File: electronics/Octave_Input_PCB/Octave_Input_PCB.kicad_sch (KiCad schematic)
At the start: 66 parts, among them J1 HRO_TYPE-C-31-M-12, SW1 SW_Hot_Swap_Socket, SW10 SW_Hot_Swap_Socket, SW11 SW_Hot_Swap_Socket, SW12 SW_Hot_Swap_Socket, SW13 SW_Hot_Swap_Socket, SW14 Alps_Alpine_RKJXV1224, SW15 Bourns_PEC12R-4xxxF-Sxxx, SW2 SW_Hot_Swap_Socket, SW21 Alps_Alpine_SKRP, SW22 Alps_Alpine_SKRP, SW3 SW_Hot_Swap_Socket, SW4 SW_Hot_Swap_Socket, SW5 SW_Hot_Swap_Socket, SW6 SW_Hot_Swap_Socket, SW7 SW_Hot_Swap_Socket, SW8 SW_Hot_Swap_Socket, SW9 SW_Hot_Swap_Socket, U1 AP2112K-3.3, U2 Raspberry_Pi_RP2040, U3 W25Q64JVSS, Y1 12MHz

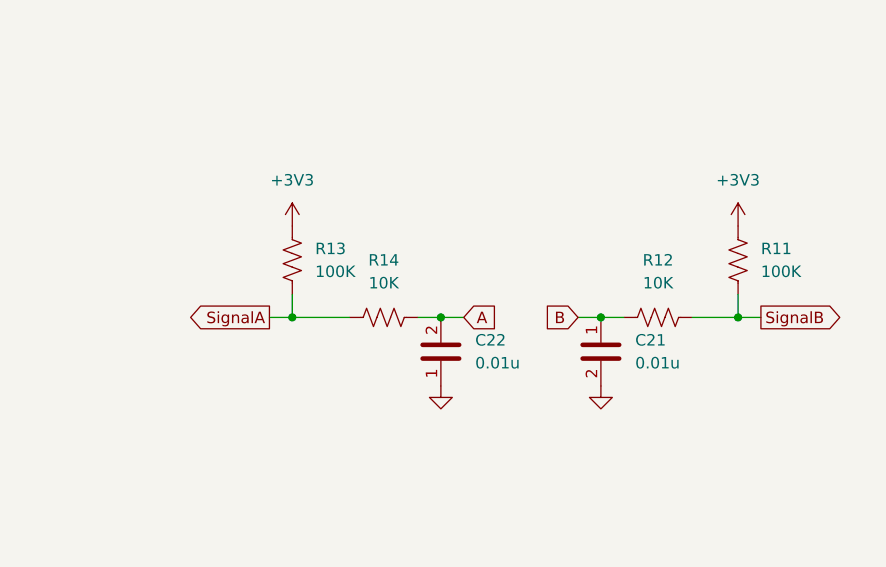
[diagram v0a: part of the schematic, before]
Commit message: [WIP] Update schematic and PCB
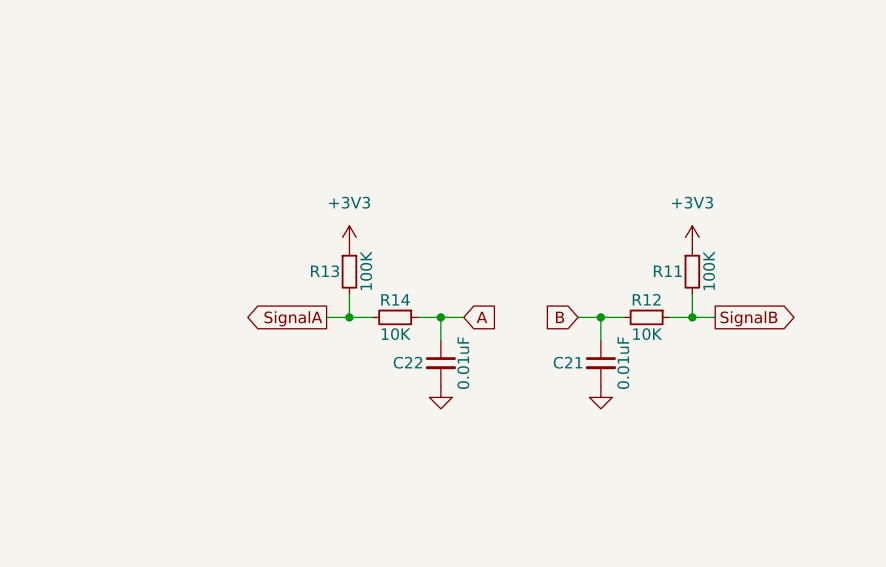
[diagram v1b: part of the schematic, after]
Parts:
- removed C21, C22: 0.01u, Octave_Library:C_0805_2012Metric, symbol Device:C
- removed R11, R13: 100K, Octave_Library:R_0805_2012Metric, symbol Device:R_US
- removed R12, R14: 10K, Octave_Library:R_0805_2012Metric, symbol Device:R_US
- added C21, C22: 0.01uF, Capacitor_SMD:C_0402_1005Metric, symbol Device:C_Small
- added R11, R13: 100K, Resistor_SMD:R_0402_1005Metric, symbol Device:R_Small
- added R12, R14: 10K, Resistor_SMD:R_0402_1005Metric, symbol Device:R_Small
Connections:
- net +3V3: now also R11.1, R13.1
- net A: now also C22.1, R14.1
- net B: now also C21.1, R12.2
- net GND: now also C21.2, C22.2
- net SignalA: now also R13.2, R14.2
- net SignalB: now also R11.2, R12.1
